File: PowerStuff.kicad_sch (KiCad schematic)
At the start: 36 parts, among them J23 UJC-HP-L-G-5-MSMT-TR, U12 TPS2117DRLR, U14 INA260AIPW, U20 AZ1117IH-3.3TRG1

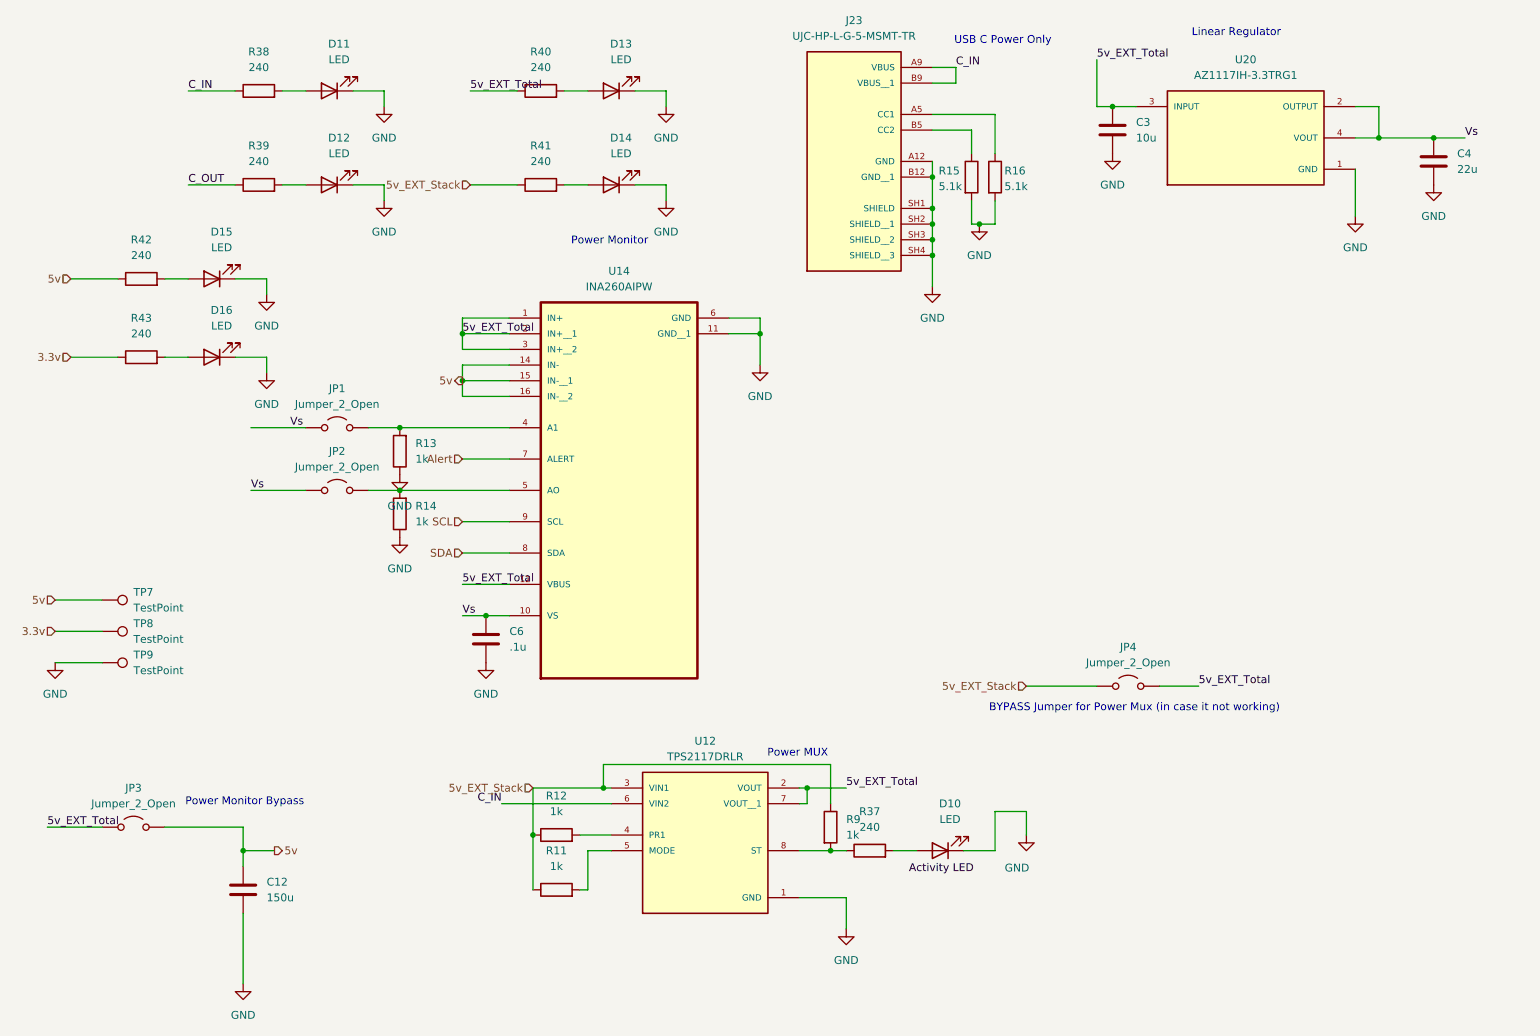
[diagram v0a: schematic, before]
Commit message: stuff
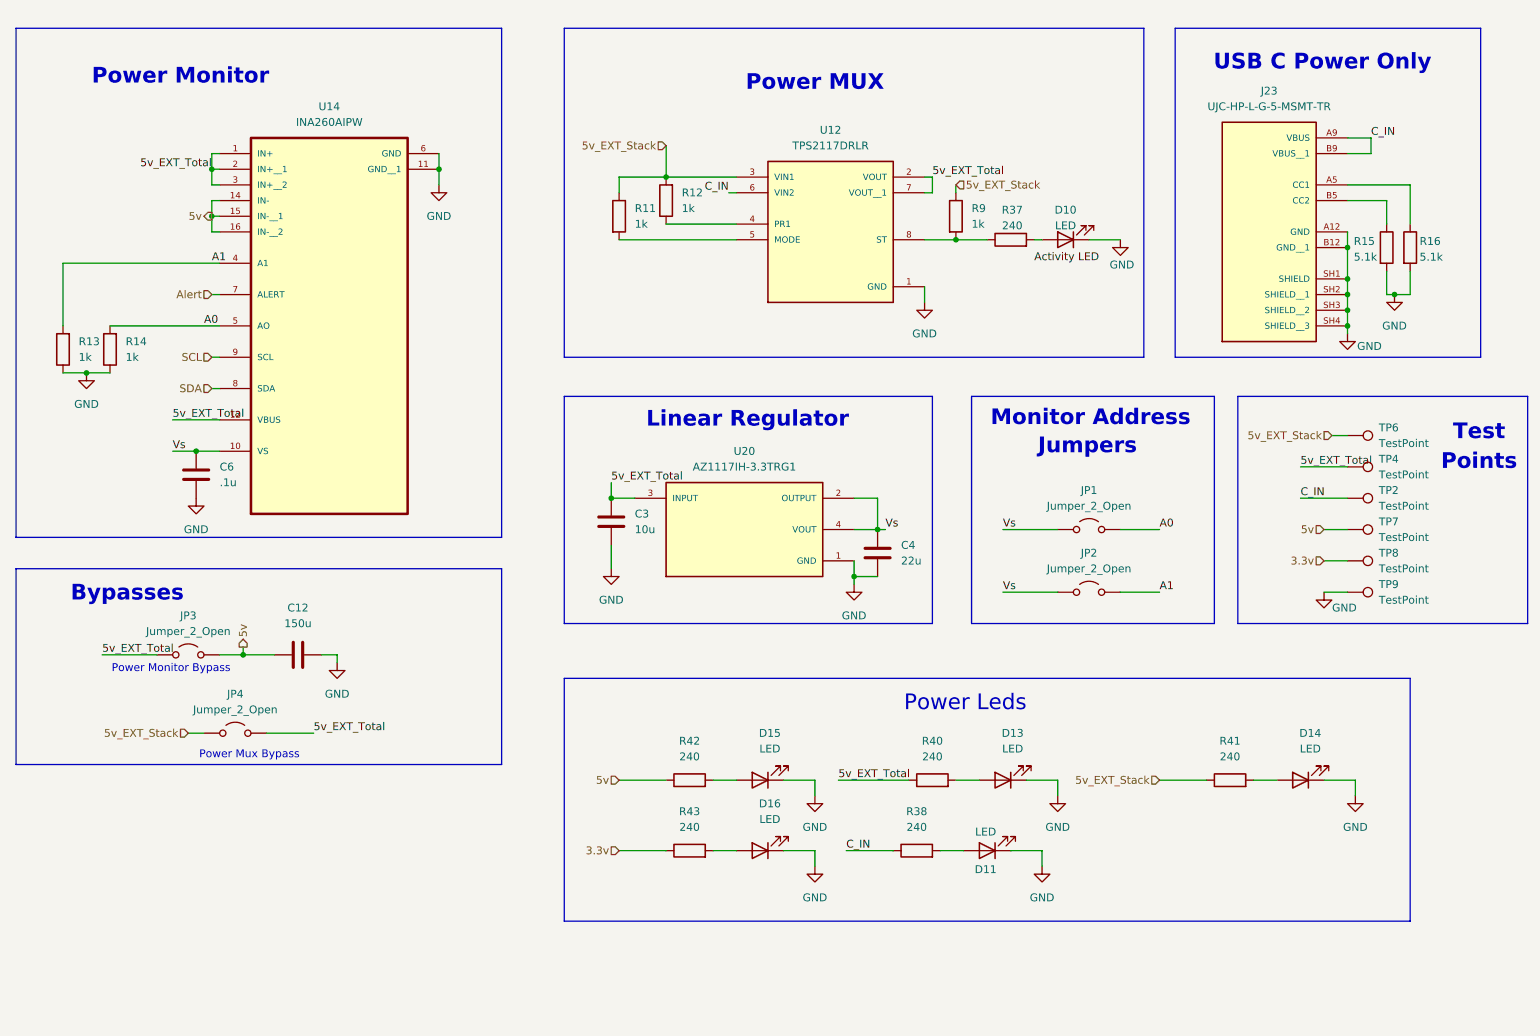
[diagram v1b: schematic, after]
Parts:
- removed D12: LED, symbol Device:LED
- removed R39: 240, symbol Device:R
- added TP2, TP4, TP6: TestPoint, symbol Connector:TestPoint
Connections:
- net 5v_EXT_Stack: now also R12.2, TP6.1; no longer R12.1
- net 5v_EXT_Total: now also TP4.1
- net C_IN: now also TP2.1
- net A1: now reaches R13.2, U14.4 (A1)
- net A1: now also JP2.2 (B); no longer JP1.2 (B)
- net A0: now reaches R14.2, U14.5 (AO)
- net A0: now also JP1.2 (B); no longer JP2.2 (B)
- net at U12.4 (PR1): now also R12.1; no longer R12.2
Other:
- note added: "Bypasses"
- note added: "Jumpers"
- note added: "Monitor Address"
- note added: "Points"
- note added: "Power Leds"
- note added: "Power Mux Bypass"
- note added: "Test"
- note removed: "BYPASS Jumper for Power Mux (in case it not working)"
- moved on the sheet: C12, C3, C4, C6, D10, D11, D13, D14, D15, D16, J23, JP1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
